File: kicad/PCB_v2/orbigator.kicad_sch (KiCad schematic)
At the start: 53 parts, among them J1 Conn_01x01, J10 Conn_01x01, J11 Conn_01x01, J12 Conn_01x01, J13 Conn_01x01, J14 Conn_01x01, J15 Conn_01x01, J16 Conn_01x01, J17 Conn_01x01, J18 Conn_01x01, J19 Conn_01x01, J2 Conn_01x01, J20 Conn_01x01, J21 Conn_01x01, J22 Conn_01x01, J23 Conn_01x01, J24 Conn_01x01, J25 Conn_01x01, J26 Conn_01x01, J27 Barrel_Jack_Switch, J28 Conn_01x01, J29 Conn_01x01, J3 Conn_01x01, J30 Conn_01x01, J32 Conn_01x01, J34 Conn_01x01, J35 Conn_01x01, J36 Conn_01x01, J37 Conn_01x01, J4 Conn_01x01, J5 Conn_01x01, J6 Conn_01x01, J7 Conn_01x01, J8 Conn_01x01, J9 Conn_01x01, M1 DYNAMIXEL_1, M2 DYNAMIXEL_2, Q1 DMG2305UX, U1 Pico_2, U2 74LS126, U4 DS3232M

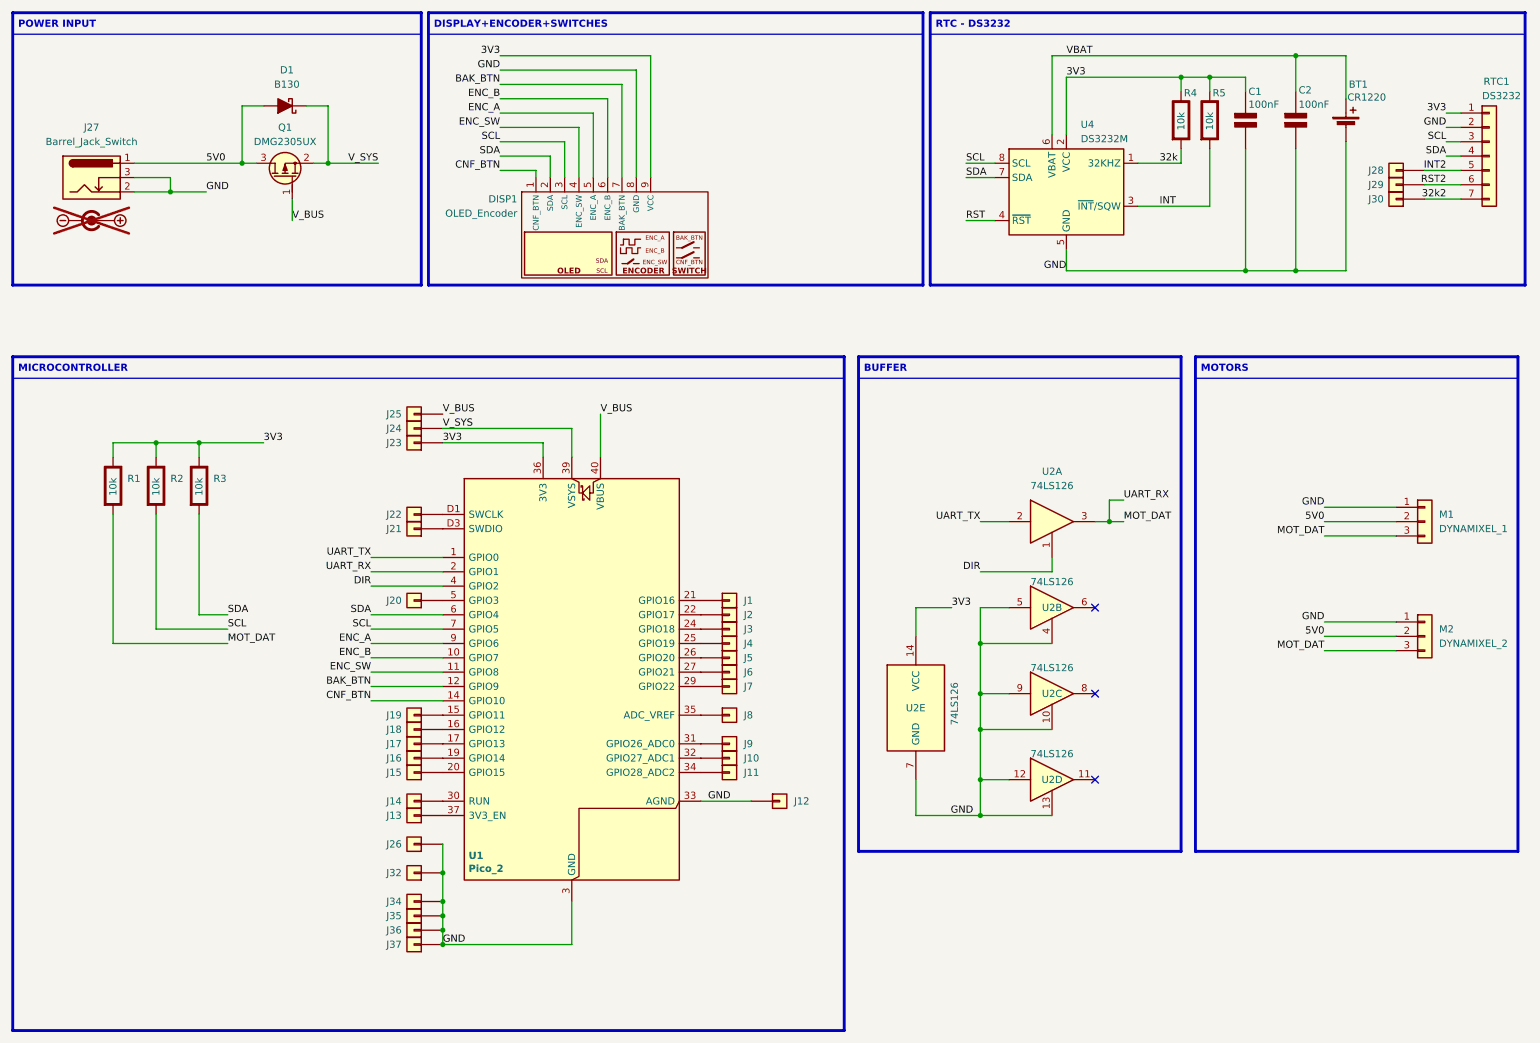
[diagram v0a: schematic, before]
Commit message: orbigator v2 WIP2 - not final yet
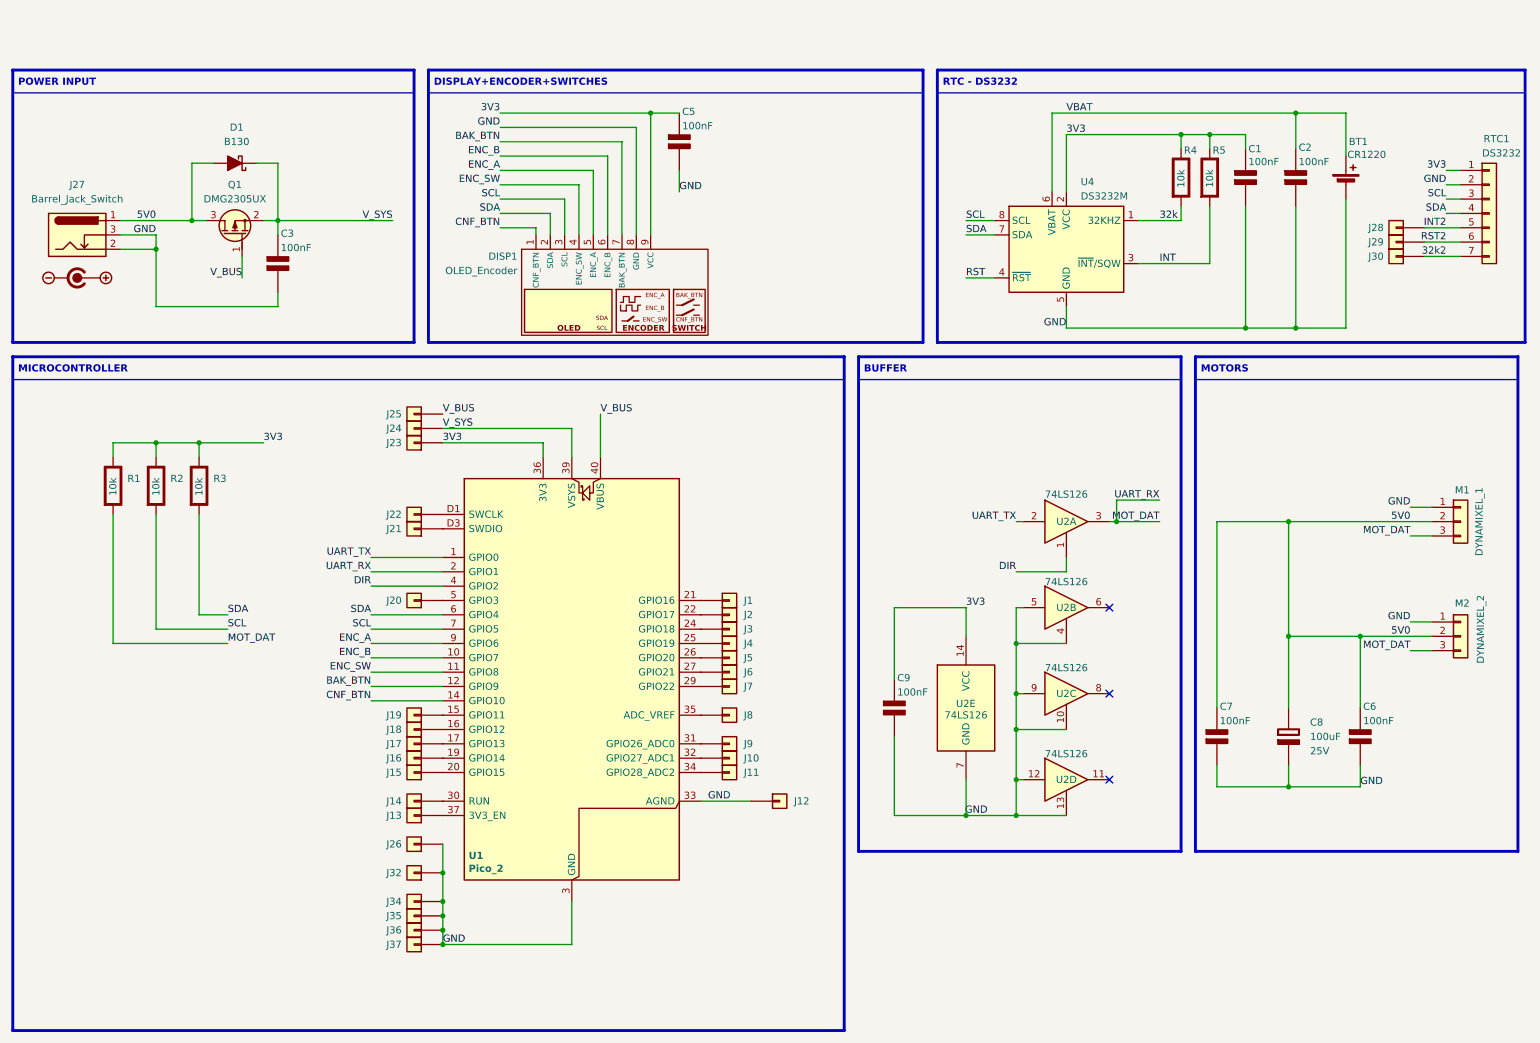
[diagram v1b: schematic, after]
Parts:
- added C3, C5, C6, C7, C9: 100nF, orbigator:C_0805_2012Metric_Pad1.18x1.45mm_HandSolder, symbol orbigator:C
- added C8: 100uF, orbigator:CP_Elec_6.3x9.9, symbol PCM_Elektuur:C-polar
- DC1: now fitted
- J10, J11, J12, J13, J14, J15, J16, J17, J18, J19, J2, J20, J21, J22, J23, J24, J25, J26, J28, J29, J3, J30, J32, J34, J35, J36, J37, J4, J5, J6, J7, J8, J9: footprint (none) -> orbigator:PinHeader_1x01_P2.54mm_Vertical
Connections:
- net 3V3: now also C5.1 (+), C9.1 (+)
- net 5V0: now also C6.1 (+), C7.1 (+), C8.1 (+)
- net GND: now also C3.2 (-), C5.2 (-), C6.2 (-), C7.2 (-), C8.2 (-), C9.2 (-)
- net V_SYS: now also C3.1 (+)
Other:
- moved on the sheet: BT1, C1, C2, D1, DISP1, J27, J28, J29, J30, M1, M2, Q1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
